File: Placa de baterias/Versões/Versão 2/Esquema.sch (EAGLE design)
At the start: 7 parts

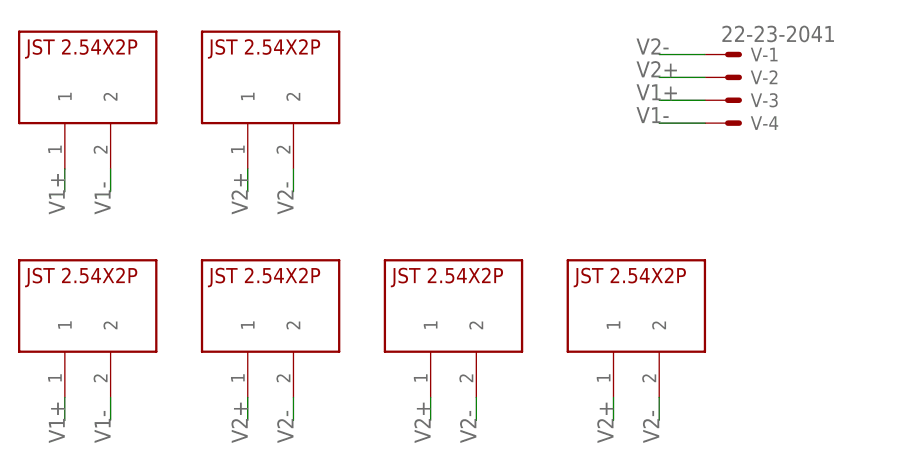
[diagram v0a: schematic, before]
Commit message: placa de baterias
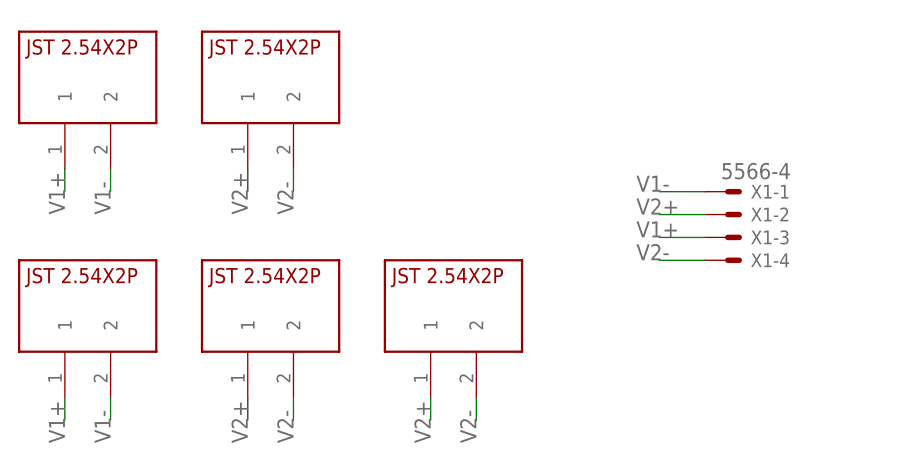
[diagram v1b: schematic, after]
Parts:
- removed U$6: JST2.54X2P, CRD:JST2.54X2P
- removed V: 22-23-2041, con-molex:22-23-2041
- added X1: 5566-4, con-molex:5566-4
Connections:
- net V1+: now also X1-3.S; no longer V-3.S
- net V1-: now also X1-1.S; no longer V-4.S
- net V2+: now also X1-2.S; no longer U$6.1, V-2.S
- net V2-: now also X1-4.S; no longer U$6.2, V-1.S
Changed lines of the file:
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@@
 <drawing>
 <settings>
-<setting alwaysvectorfont="yes"/>
+<setting alwaysvectorfont="no"/>
 <setting verticaltext="up"/>
 </settings>
@@
 <part name="U$4" library="CRD" library_urn="urn:adsk.eagle:library:39051337" deviceset="JST2.54X2P" device="" package3d_urn="urn:adsk.eagle:package:39191967/2"/>
 <part name="U$5" library="CRD" library_urn="urn:adsk.eagle:library:39051337" deviceset="JST2.54X2P" device="" package3d_urn="urn:adsk.eagle:package:39191967/2"/>
-<part name="V" library="con-molex" library_urn="urn:adsk.eagle:library:165" deviceset="22-23-2041" device="" package3d_urn="urn:adsk.eagle:package:8078635/1"/>
-<part name="U$6" library="CRD" library_urn="urn:adsk.eagle:library:39051337" deviceset="JST2.54X2P" device="" package3d_urn="urn:adsk.eagle:package:39191967/2"/>
+<part name="X1" library="con-molex" library_urn="urn:adsk.eagle:library:165" deviceset="5566-4" device="" package3d_urn="urn:adsk.eagle:package:8078582/1"/>
 </parts>
 <sheets>
@@
 <instance part="U$4" gate="G$1" x="-20.32" y="25.4" smashed="yes"/>
 <instance part="U$5" gate="G$1" x="0" y="25.4" smashed="yes"/>
-<instance part="V" gate="-1" x="50.8" y="27.94" smashed="yes">
-<attribute name="NAME" x="53.34" y="27.178" size="1.524" layer="95"/>
-<attribute name="VALUE" x="50.038" y="29.337" size="1.778" layer="96"/>
+<instance part="X1" gate="-1" x="50.8" y="12.7" smashed="yes">
+<attribute name="NAME" x="53.34" y="11.938" size="1.524" layer="95"/>
+<attribute name="VALUE" x="50.038" y="14.097" size="1.778" layer="96"/>
 </instance>
-<instance part="V" gate="-2" x="50.8" y="25.4" smashed="yes">
-<attribute name="NAME" x="53.34" y="24.638" size="1.524" layer="95"/>
+<instance part="X1" gate="-2" x="50.8" y="10.16" smashed="yes">
+<attribute name="NAME" x="53.34" y="9.398" size="1.524" layer="95"/>
 </instance>
-<instance part="V" gate="-3" x="50.8" y="22.86" smashed="yes">
-<attribute name="NAME" x="53.34" y="22.098" size="1.524" layer="95"/>
+<instance part="X1" gate="-3" x="50.8" y="7.62" smashed="yes">
+<attribute name="NAME" x="53.34" y="6.858" size="1.524" layer="95"/>
 </instance>
-<instance part="V" gate="-4" x="50.8" y="20.32" smashed="yes">
-<attribute name="NAME" x="53.34" y="19.558" size="1.524" layer="95"/>
+<instance part="X1" gate="-4" x="50.8" y="5.08" smashed="yes">
+<attribute name="NAME" x="53.34" y="4.318" size="1.524" layer="95"/>
 </instance>
-<instance part="U$6" gate="G$1" x="40.64" y="0" smashed="yes"/>
 </instances>
 <busses>
@@
 </segment>
 <segment>
-<pinref part="V" gate="-3" pin="S"/>
-<wire x1="48.26" y1="22.86" x2="43.18" y2="22.86" width="0.1524" layer="91"/>
-<label x="40.64" y="22.86" size="1.778" layer="95"/>
+<pinref part="X1" gate="-3" pin="S"/>
+<wire x1="48.26" y1="7.62" x2="43.18" y2="7.62" width="0.1524" layer="91"/>
+<label x="40.64" y="7.62" size="1.778" layer="95"/>
 </segment>
 </net>
@@
 </segment>
 <segment>
-<pinref part="V" gate="-4" pin="S"/>
-<wire x1="48.26" y1="20.32" x2="43.18" y2="20.32" width="0.1524" layer="91"/>
-<label x="40.64" y="20.32" size="1.778" layer="95"/>
+<pinref part="X1" gate="-1" pin="S"/>
+<wire x1="48.26" y1="12.7" x2="43.18" y2="12.7" width="0.1524" layer="91"/>
+<label x="40.64" y="12.7" size="1.778" layer="95"/>
 </segment>
 </net>
@@
 </segment>
 <segment>
-<pinref part="V" gate="-2" pin="S"/>
-<wire x1="48.26" y1="25.4" x2="43.18" y2="25.4" width="0.1524" layer="91"/>
-<label x="40.64" y="25.4" size="1.778" layer="95"/>
-</segment>
-<segment>
-<pinref part="U$6" gate="G$1" pin="1"/>
-<wire x1="38.1" y1="-10.16" x2="38.1" y2="-12.7" width="0.1524" layer="91"/>
-<label x="38.1" y="-15.24" size="1.778" layer="95" rot="R90"/>
+<pinref part="X1" gate="-2" pin="S"/>
+<wire x1="48.26" y1="10.16" x2="43.18" y2="10.16" width="0.1524" layer="91"/>
+<label x="40.64" y="10.16" size="1.778" layer="95"/>
 </segment>
 </net>
@@
 </segment>
 <segment>
-<pinref part="V" gate="-1" pin="S"/>
-<wire x1="48.26" y1="27.94" x2="43.18" y2="27.94" width="0.1524" layer="91"/>
-<label x="40.64" y="27.94" size="1.778" layer="95"/>
-</segment>
-<segment>
-<pinref part="U$6" gate="G$1" pin="2"/>
-<wire x1="43.18" y1="-10.16" x2="43.18" y2="-12.7" width="0.1524" layer="91"/>
-<label x="43.18" y="-15.24" size="1.778" layer="95" rot="R90"/>
+<pinref part="X1" gate="-4" pin="S"/>
+<wire x1="48.26" y1="5.08" x2="43.18" y2="5.08" width="0.1524" layer="91"/>
+<label x="40.64" y="5.08" size="1.778" layer="95"/>
 </segment>
 </net>
